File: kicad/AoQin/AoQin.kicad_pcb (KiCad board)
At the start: 2 copper layers, 111.2 x 81 mm, 17 parts, among them J1 Conn_01x03_Socket, J10 1985218, J12 1985218, J2 Conn_01x03_Socket, J3 Conn_02x03_Odd_Even, J4 Conn_02x03_Odd_Even, J5 1985218, J6 1985218, J8 1985218, J9 1985218

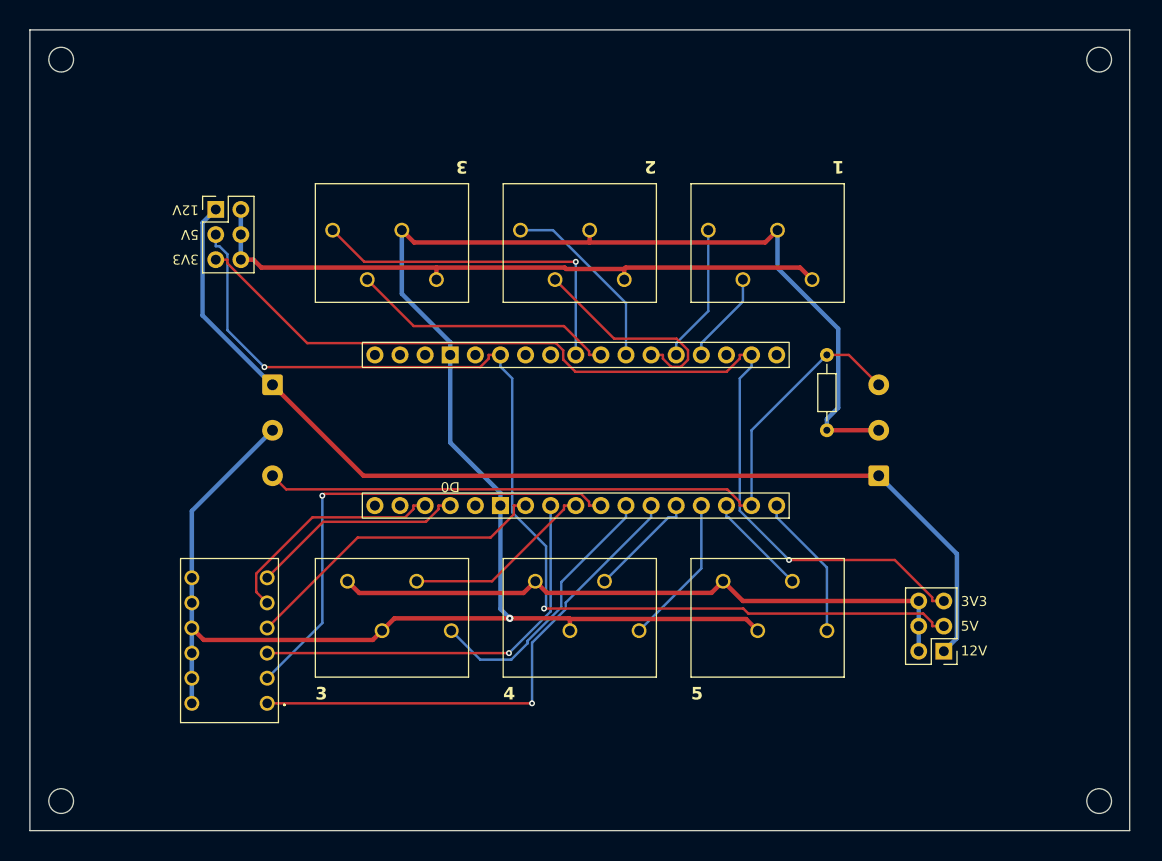
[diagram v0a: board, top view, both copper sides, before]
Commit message: The King of Assassins
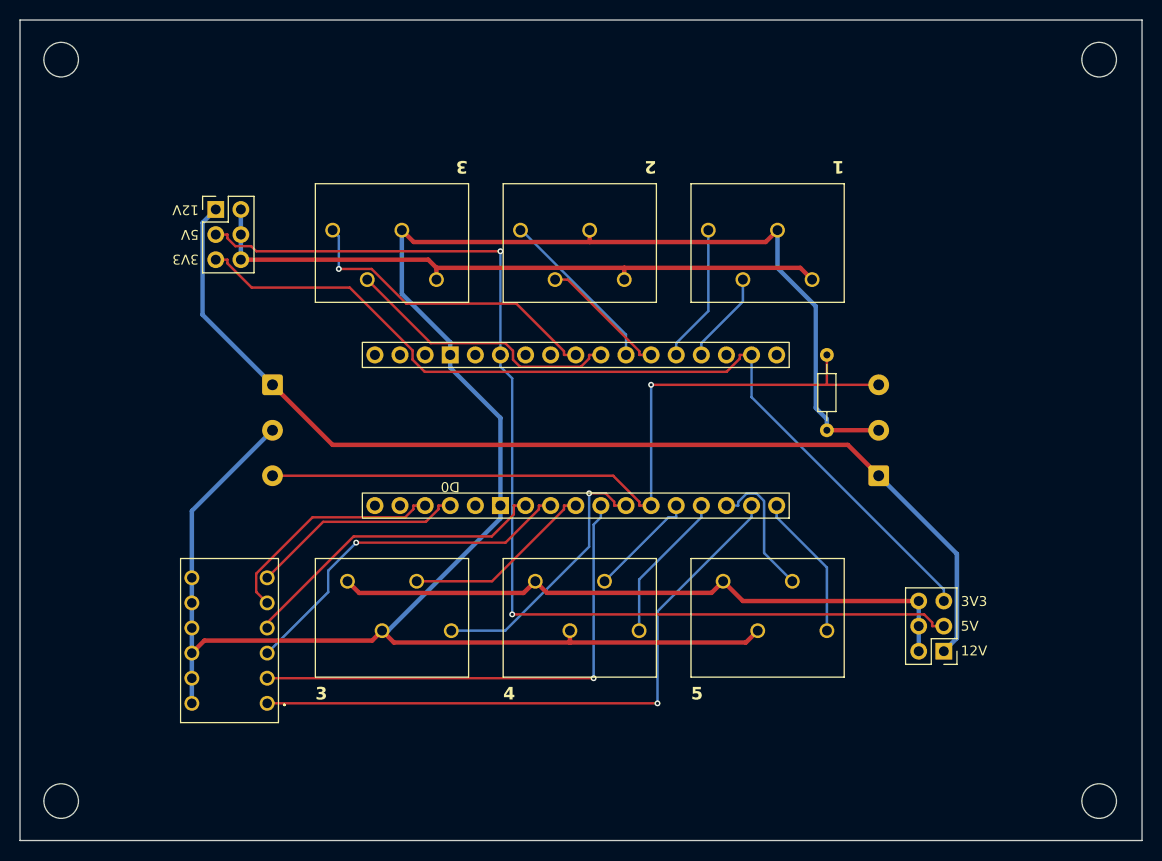
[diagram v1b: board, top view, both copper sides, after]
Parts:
- removed H1, H2, H3, H4: MountingHole_2.5mm, MountingHole:MountingHole_2.5mm
- added M1: MountingHole_3.5mm, MountingHole:MountingHole_3.5mm, F.Cu at (35.5, 95.5)
- added M2: MountingHole_3.5mm, MountingHole:MountingHole_3.5mm, F.Cu at (140.5, 95.5)
- added M3: MountingHole_3.5mm, MountingHole:MountingHole_3.5mm, F.Cu at (140.5, 20.5)
- added M4: MountingHole_3.5mm, MountingHole:MountingHole_3.5mm, F.Cu at (35.5, 20.5)
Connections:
- J1 pad 3: /D11 -> /D7
- J2 pad 3: /D11 -> /D7
- R13 pad 1: /D11 -> /D7
- S2 pad 1: /D7 -> /D11
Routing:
- net /D7: track 51.8 -> 78.0 mm
- net /D11: track 74.8 -> 63.4 mm, vias 0 -> 1
- net /A2: track 22.1 -> 13.1 mm
- net /3V3: track 101.5 -> 93.5 mm, vias 1 -> 0
- net GND: track 203.9 -> 209.1 mm, vias 1 -> 0
- net /D3: track 41.1 -> 36.3 mm
- net /A10: track 10.5 -> 14.1 mm
- net /A5: track 35.3 -> 32.0 mm
- net /5V: track 109.3 -> 111.3 mm
- net /A3: track 19.0 -> 17.1 mm
- net /A4: track 27.0 -> 28.5 mm
- net /D5: track 49.7 -> 50.8 mm
- net /A7: track 27.7 -> 27.3 mm, vias 0 -> 1
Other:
- board size 111.2 x 81 mm -> 113.5 x 83 mm
